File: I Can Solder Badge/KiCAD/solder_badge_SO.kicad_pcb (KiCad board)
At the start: 2 copper layers, 44.9 x 44.8 mm, 11 parts

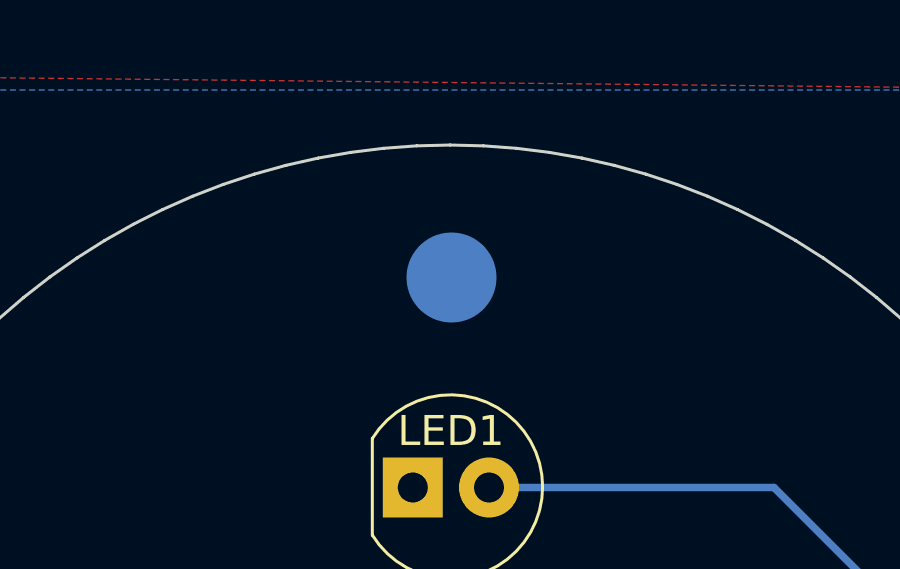
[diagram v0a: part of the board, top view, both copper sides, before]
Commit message: Updated files
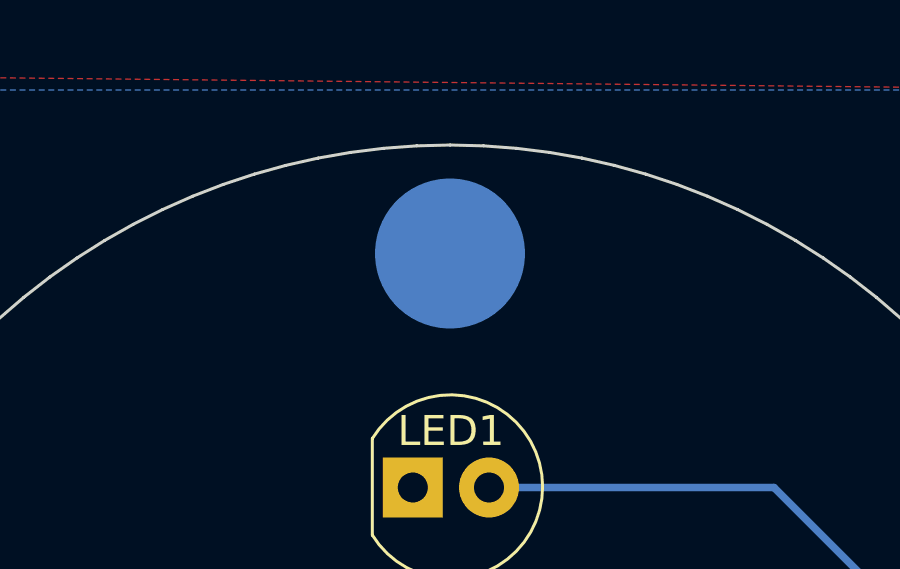
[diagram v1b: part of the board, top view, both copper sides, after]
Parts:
- moved Pin: 0.80 mm to (229.0, 119.3)
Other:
- rule pad_to_mask_clearance: 0.2 -> 0
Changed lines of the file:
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@@
 	)
 	(setup
-		(pad_to_mask_clearance 0.2)
+		(pad_to_mask_clearance 0)
 		(allow_soldermask_bridges_in_footprints no)
 		(pcbplotparams
-			(layerselection 0x00010f0_80000001)
+			(layerselection 0x00010f0_ffffffff)
 			(plot_on_all_layers_selection 0x0000000_00000000)
 			(disableapertmacros no)
@@
 	(footprint "solder-badge-SO:pad"
 		(layer "B.Cu")
-		(at 229.05 120.1)
+		(at 229 119.3)
 		(property "Reference" "Pin:"
-			(at 3.5 0 0)
+			(at 4.4 0 0)
 			(layer "B.SilkS")
 			(effects
@@
 		(pad "1" smd circle
 			(at 0 0)
-			(size 3 3)
+			(size 5 5)
 			(layers "B.Cu" "B.Paste" "B.Mask")
 		)
